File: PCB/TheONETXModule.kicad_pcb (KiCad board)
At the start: 2 copper layers, 41 x 56 mm, 23 parts, among them J1 TX_IN, SW1 Bind Button, T1 A7105-Hubsan, U1 L7805, U2 LD1117S33, U3 NRF24L01, U4 4ChLogicShift

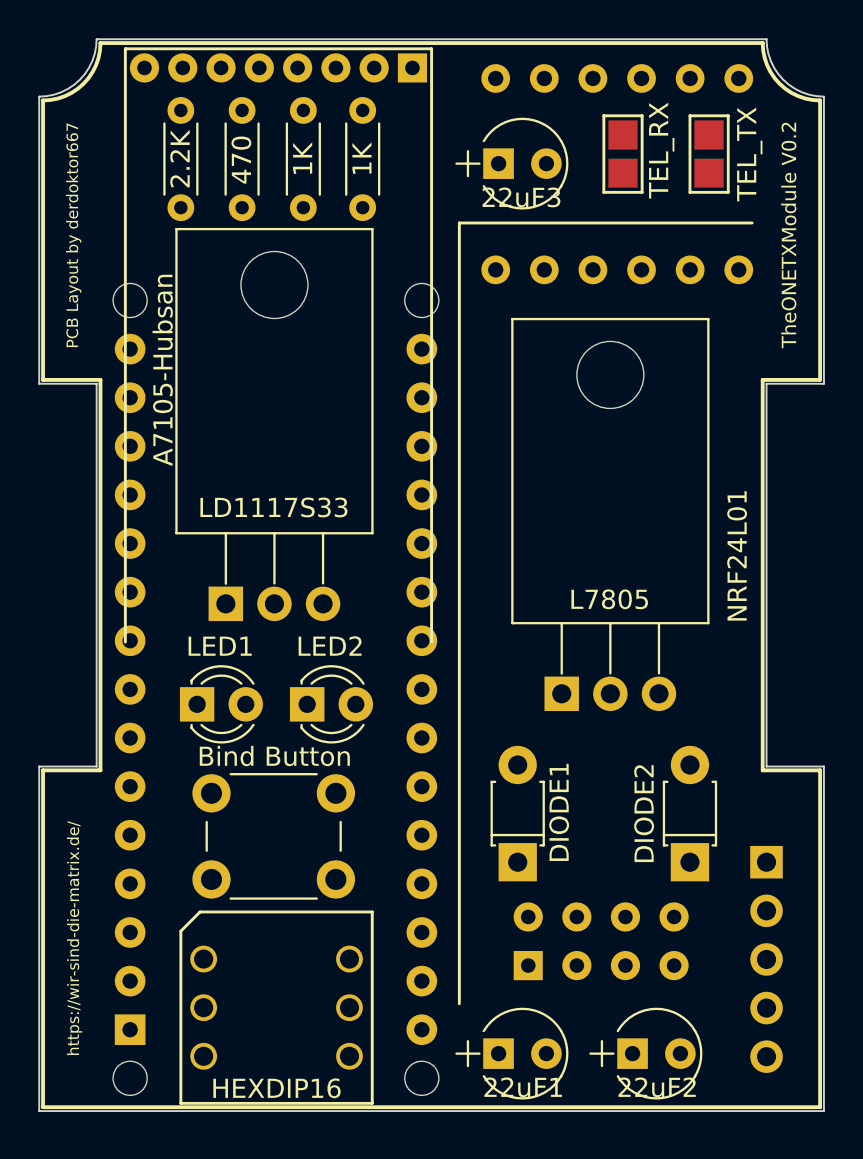
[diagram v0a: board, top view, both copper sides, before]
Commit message: ...bump
...bump
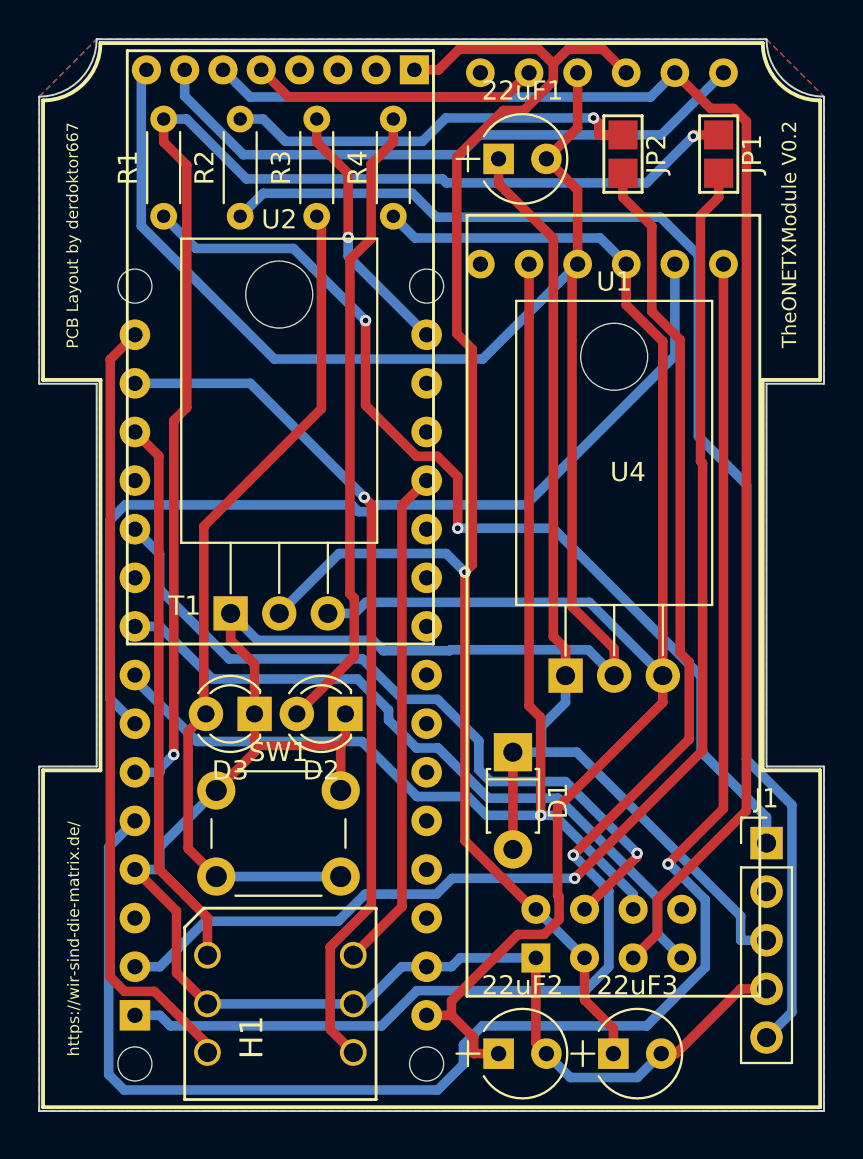
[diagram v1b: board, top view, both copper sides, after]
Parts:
- removed DIODE1, DIODE2: D, Diodes_THT:D_T-1_P5.08mm_Horizontal
- removed G***: LOGO, temp:test
- added D3: LED, LEDs:LED_D3.0mm, F.Cu at (128.2, 108.2)
- A1: value Arduino Nano v3.2 -> Arduino_Nano_v3.x
- D1: value LED1 -> D; footprint LEDs:LED_D3.0mm -> Diodes_THT:D_T-1_P5.08mm_Horizontal
- D2: value LED2 -> LED
- H1: value HEXDIP16 -> HEX_CODER_16
- J1: value TX_IN -> Conn_01x05_Female; moved to F.Cu
- U3: value NRF24L01 -> LogicShift; footprint customs:NRF24L01_PA -> customs:4Ch-LogicShift; moved to B.Cu
- U4: value 4ChLogicShift -> NRF24L01; footprint customs:4Ch-LogicShift -> customs:NRF24L01_PA; moved to F.Cu
- moved 22uF3 46.9 mm to (147.0, 126.0)
- moved 22uF1 46.8 mm to (141.0, 79.2)
- moved U3 43.4 mm to (146.0, 80.0)
- moved U4 43.2 mm to (147.0, 123.0), turned to 0 degrees
- moved D1 16.7 mm to (141.8, 110.2), turned to 270 degrees
- moved JP2 8.50 mm to (145.5, 79.0), turned to 270 degrees
- moved 22uF2 7.00 mm to (141.0, 126.0)
- moved D2 2.06 mm to (133.0, 108.2), turned to 180 degrees
- moved R4 1.66 mm to (135.5, 82.2)
- moved R1 1.01 mm to (123.5, 82.2)
- moved J1 1.00 mm to (155.0, 115.0), turned to 0 degrees
- moved JP1 1.00 mm to (150.5, 79.0), turned to 270 degrees
- moved U1 0.97 mm to (144.5, 106.2)
- moved R3 0.83 mm to (131.5, 82.2)
- moved A1 0.79 mm to (122.0, 124.0)
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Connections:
- D1 pad 1: GND -> /VBAT+
- D1 pad 2: Net-(D1-Pad2) -> /VBAT+
- R1 pad 2: Net-(D3-Pad2) -> /PPM_IN
- R3 pad 1: Net-(D2-Pad2) -> Net-(D3-Pad2)
- R4 pad 2: Net-(D1-Pad2) -> Net-(D2-Pad2)
- SW1 pad 2: Net-(D2-Pad2) -> Net-(D3-Pad2)
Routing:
- net GND: track 0.00 -> 163.1 mm
- net /A7105_CS: track 0.00 -> 87.4 mm, vias 0 -> 1
- net /5V: track 0.00 -> 83.1 mm
- net /3.3V: track 0.00 -> 82.3 mm, vias 0 -> 1
- net /SCK_LV: track 0.00 -> 75.7 mm
- net /TX_IN: track 0.00 -> 72.4 mm, vias 0 -> 1
- net Net-(J1-Pad5): track 0.00 -> 69.2 mm
- net /PPM_IN: track 0.00 -> 67.9 mm, vias 0 -> 2
- net /RX_IN: track 0.00 -> 64.9 mm, vias 0 -> 1
- net /MOSI: track 0.00 -> 60.8 mm, vias 0 -> 1
- net /VBAT+: track 0.00 -> 56.1 mm
- net /PPM: track 0.00 -> 52.3 mm, vias 0 -> 2
- net /SCK: track 0.00 -> 49.3 mm
- net /D11: track 0.00 -> 45.0 mm, vias 0 -> 1
- net Net-(D3-Pad2): track 0.00 -> 44.7 mm
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- added copper zone on B.Cu, net GND
- added copper zone on F.Cu, net GND
